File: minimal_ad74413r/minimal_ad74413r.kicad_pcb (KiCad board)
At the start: 4 copper layers, 30.5 x 25.4 mm, 17 parts, among them U8 AD74413RBCPZ

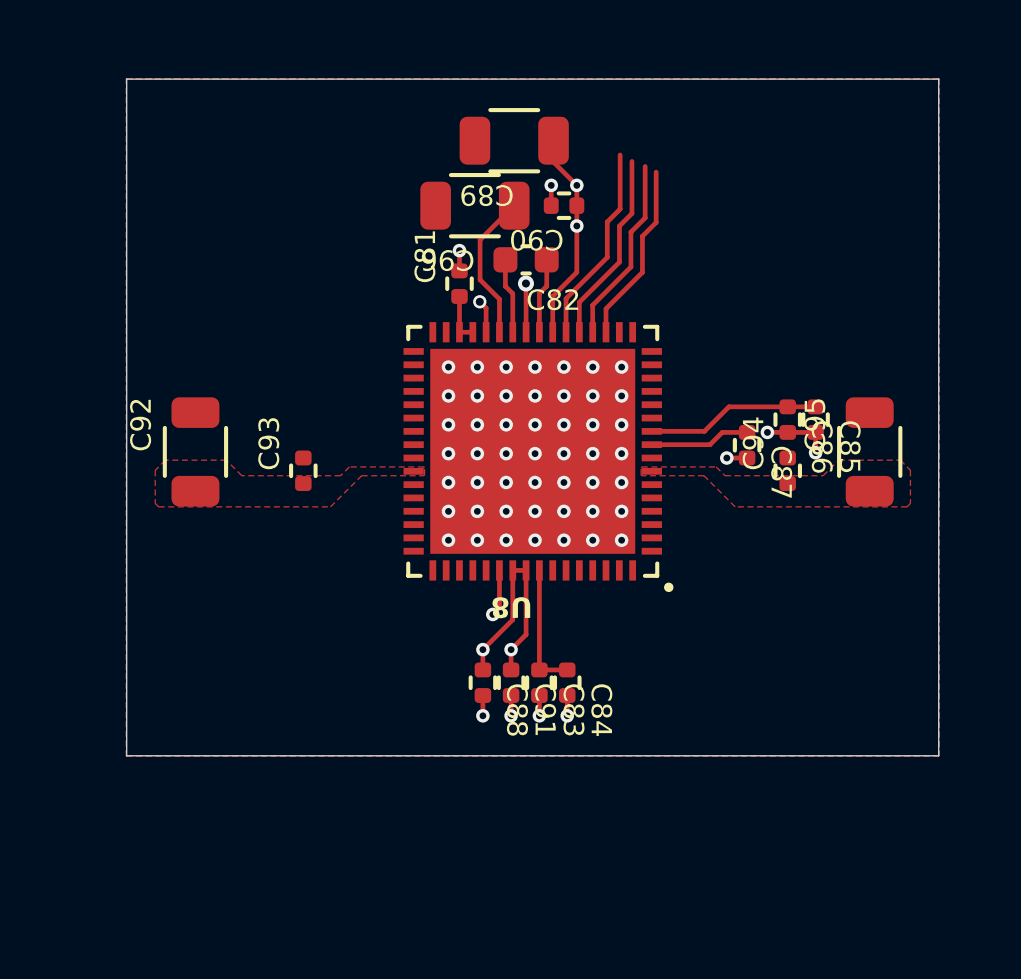
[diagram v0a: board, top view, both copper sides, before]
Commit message: backup
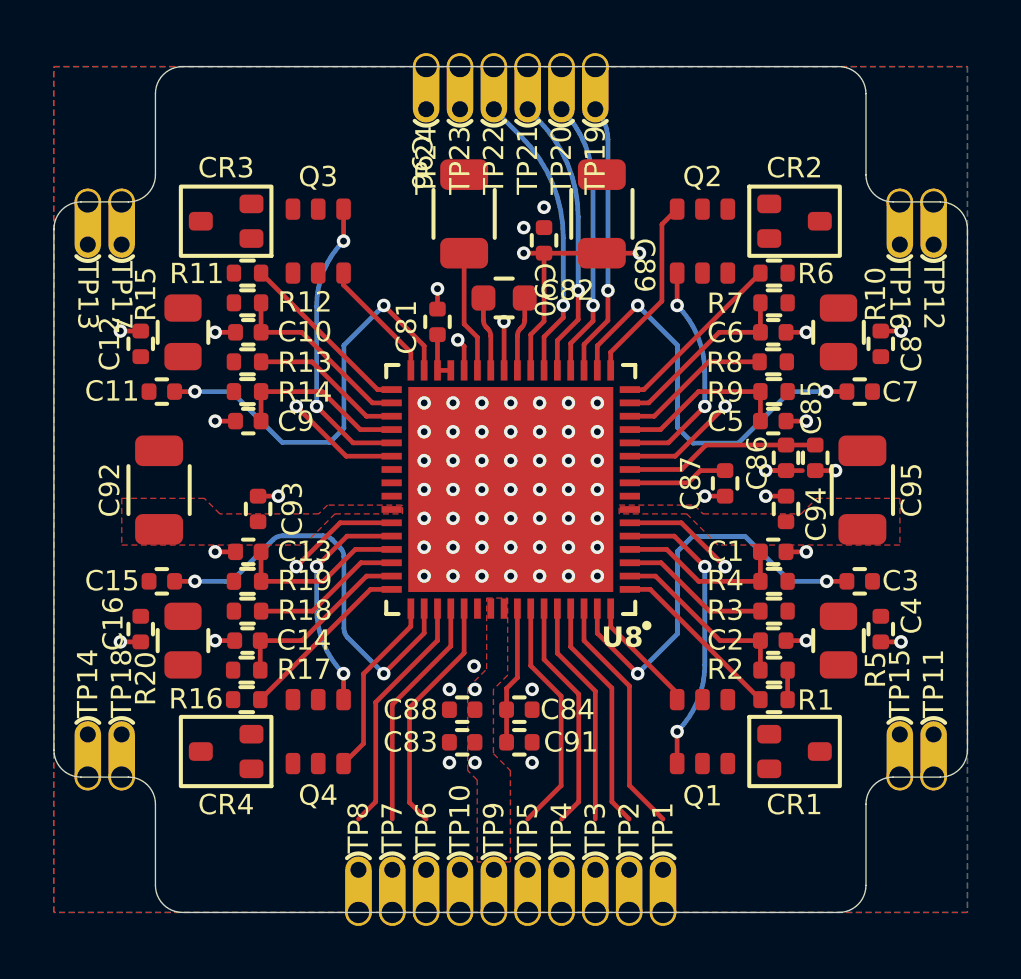
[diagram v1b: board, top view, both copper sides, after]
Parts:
- added C1: 0.01 uF, capacitor_footprints:C_0402_1005Metric, F.Cu at (161.6, 105.2)
- added C10: 0.01 uF, capacitor_footprints:C_0402_1005Metric, F.Cu at (141.9, 97.0)
- added C11: 220 pF, capacitor_footprints:C_0402_1005Metric, F.Cu at (138.7, 99.2)
- added C12: 0.01 uF, capacitor_footprints:C_0402_1005Metric, F.Cu at (137.9, 97.4)
- added C13: 0.01 uF, capacitor_footprints:C_0402_1005Metric, F.Cu at (141.9, 105.2)
- added C14: 0.01 uF, capacitor_footprints:C_0402_1005Metric, F.Cu at (141.9, 108.5)
- added C15: 220 pF, capacitor_footprints:C_0402_1005Metric, F.Cu at (138.7, 106.3)
- added C16: 0.01 uF, capacitor_footprints:C_0402_1005Metric, F.Cu at (137.9, 108.1)
- added C2: 0.01 uF, capacitor_footprints:C_0402_1005Metric, F.Cu at (161.6, 108.5)
- added C3: 220 pF, capacitor_footprints:C_0402_1005Metric, F.Cu at (164.9, 106.3)
- added C4: 0.01 uF, capacitor_footprints:C_0402_1005Metric, F.Cu at (165.7, 108.1)
- added C5: 0.01 uF, capacitor_footprints:C_0402_1005Metric, F.Cu at (161.6, 100.3)
- added C6: 0.01 uF, capacitor_footprints:C_0402_1005Metric, F.Cu at (161.6, 97.0)
- added C7: 220 pF, capacitor_footprints:C_0402_1005Metric, F.Cu at (164.9, 99.2)
- added C8: 0.01 uF, capacitor_footprints:C_0402_1005Metric, F.Cu at (165.7, 97.4)
- added C9: 0.01 uF, capacitor_footprints:C_0402_1005Metric, F.Cu at (141.9, 100.3)
- added CR1: SBAV99WT1G, diode_footprints:SC_70, F.Cu at (162.4, 112.7)
- added CR2: SBAV99WT1G, diode_footprints:SC_70, F.Cu at (162.4, 92.8)
- added CR3: SBAV99WT1G, diode_footprints:SC_70, F.Cu at (141.1, 92.8)
- added CR4: SBAV99WT1G, diode_footprints:SC_70, F.Cu at (141.1, 112.7)
- added Q1: ZXMP6A17E6TA, transistor_footprints:SOT-26, F.Cu at (159.0, 112.0)
- added Q2: ZXMP6A17E6TA, transistor_footprints:SOT-26, F.Cu at (159.0, 93.5)
- added Q3: ZXMP6A17E6TA, transistor_footprints:SOT-26, F.Cu at (144.5, 93.5)
- added Q4: ZXMP6A17E6TA, transistor_footprints:SOT-26, F.Cu at (144.5, 112.0)
- added R1: 2k, resistor_footprints:R_0402_1005Metric, F.Cu at (161.6, 110.8)
- added R10: 100, resistor_footprints:R_0805_2012Metric, F.Cu at (164.1, 97.0)
- added R11: 2k, resistor_footprints:R_0402_1005Metric, F.Cu at (141.9, 94.7)
- added R12: 10k, resistor_footprints:R_0402_1005Metric, F.Cu at (141.9, 95.9)
- added R13: 2k, resistor_footprints:R_0402_1005Metric, F.Cu at (141.9, 98.1)
- added R14: 10k, resistor_footprints:R_0402_1005Metric, F.Cu at (141.9, 99.2)
- added R15: 100, resistor_footprints:R_0805_2012Metric, F.Cu at (139.5, 97.0)
- added R16: 2k, resistor_footprints:R_0402_1005Metric, F.Cu at (141.9, 110.8)
- added R17: 10k, resistor_footprints:R_0402_1005Metric, F.Cu at (141.9, 109.6)
- added R18: 2k, resistor_footprints:R_0402_1005Metric, F.Cu at (141.9, 107.4)
- added R19: 10k, resistor_footprints:R_0402_1005Metric, F.Cu at (141.9, 106.3)
- added R2: 10k, resistor_footprints:R_0402_1005Metric, F.Cu at (161.6, 109.6)
- added R20: 100, resistor_footprints:R_0805_2012Metric, F.Cu at (139.5, 108.5)
- added R3: 2k, resistor_footprints:R_0402_1005Metric, F.Cu at (161.6, 107.4)
- added R4: 10k, resistor_footprints:R_0402_1005Metric, F.Cu at (161.6, 106.3)
- added R5: 100, resistor_footprints:R_0805_2012Metric, F.Cu at (164.1, 108.5)
- added R6: 2k, resistor_footprints:R_0402_1005Metric, F.Cu at (161.6, 94.7)
- added R7: 10k, resistor_footprints:R_0402_1005Metric, F.Cu at (161.6, 95.9)
- added R8: 2k, resistor_footprints:R_0402_1005Metric, F.Cu at (161.6, 98.1)
- added R9: 10k, resistor_footprints:R_0402_1005Metric, F.Cu at (161.6, 99.2)
- added TP1: TestPoint, test_point_footprints:TestPoint_THTPad_Castelated, F.Cu at (157.5, 118.7)
- added TP10: TestPoint, test_point_footprints:TestPoint_THTPad_Castelated, F.Cu at (149.9, 118.7)
- added TP11: TestPoint, test_point_footprints:TestPoint_THTPad_Castelated, F.Cu at (167.6, 113.7)
- added TP12: TestPoint, test_point_footprints:TestPoint_THTPad_Castelated, F.Cu at (167.6, 92.1)
- added TP13: TestPoint, test_point_footprints:TestPoint_THTPad_Castelated, F.Cu at (135.9, 92.1)
- added TP14: TestPoint, test_point_footprints:TestPoint_THTPad_Castelated, F.Cu at (135.9, 113.7)
- added TP15: TestPoint, test_point_footprints:TestPoint_THTPad_Castelated, F.Cu at (166.4, 113.7)
- added TP16: TestPoint, test_point_footprints:TestPoint_THTPad_Castelated, F.Cu at (166.4, 92.1)
- added TP17: TestPoint, test_point_footprints:TestPoint_THTPad_Castelated, F.Cu at (137.2, 92.1)
- added TP18: TestPoint, test_point_footprints:TestPoint_THTPad_Castelated, F.Cu at (137.2, 113.7)
- added TP19: TestPoint, test_point_footprints:TestPoint_THTPad_Castelated, F.Cu at (154.9, 87.0)
- added TP2: TestPoint, test_point_footprints:TestPoint_THTPad_Castelated, F.Cu at (156.2, 118.7)
- added TP20: TestPoint, test_point_footprints:TestPoint_THTPad_Castelated, F.Cu at (153.7, 87.0)
- added TP21: TestPoint, test_point_footprints:TestPoint_THTPad_Castelated, F.Cu at (152.4, 87.0)
- added TP22: TestPoint, test_point_footprints:TestPoint_THTPad_Castelated, F.Cu at (151.1, 87.0)
- added TP23: TestPoint, test_point_footprints:TestPoint_THTPad_Castelated, F.Cu at (149.9, 87.0)
- added TP24: TestPoint, test_point_footprints:TestPoint_THTPad_Castelated, F.Cu at (148.6, 87.0)
- added TP3: TestPoint, test_point_footprints:TestPoint_THTPad_Castelated, F.Cu at (154.9, 118.7)
- added TP4: TestPoint, test_point_footprints:TestPoint_THTPad_Castelated, F.Cu at (153.7, 118.7)
- added TP5: TestPoint, test_point_footprints:TestPoint_THTPad_Castelated, F.Cu at (152.4, 118.7)
- added TP6: TestPoint, test_point_footprints:TestPoint_THTPad_Castelated, F.Cu at (148.6, 118.7)
- added TP7: TestPoint, test_point_footprints:TestPoint_THTPad_Castelated, F.Cu at (147.3, 118.7)
- added TP8: TestPoint, test_point_footprints:TestPoint_THTPad_Castelated, F.Cu at (146.1, 118.7)
- added TP9: TestPoint, test_point_footprints:TestPoint_THTPad_Castelated, F.Cu at (151.1, 118.7)
- C82: footprint footprints:C_0603_1608Metric -> capacitor_footprints:C_0603_1608Metric
- moved C89 4.29 mm to (155.2, 92.5), turned to 90 degrees
- moved C91 2.89 mm to (149.9, 112.4), turned to 180 degrees
- moved C83 2.36 mm to (152.1, 112.4), turned to 0 degrees
- moved C93 2.22 mm to (142.3, 103.6)
- moved C84 2.06 mm to (152.1, 111.1), turned to 0 degrees
- moved C92 1.98 mm to (138.6, 102.9)
- moved U8 1.65 mm to (151.8, 102.9)
- moved C81 1.65 mm to (149.0, 96.6)
- moved C82 1.65 mm to (151.5, 95.7)
- moved C87 1.65 mm to (159.8, 102.6)
- moved C90 1.50 mm to (153.0, 93.5), turned to 90 degrees
- moved C95 1.46 mm to (165.0, 102.9)
- moved C86 1.43 mm to (162.1, 101.7)
- moved C94 1.43 mm to (162.1, 103.6)
- moved C85 1.43 mm to (163.2, 101.7)
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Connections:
- C88 pad 1: (no net) -> /3V3
- C89 pad 1: /3V3_ISO -> /3V3
- C90 pad 1: /3V3_ISO -> /3V3
- C91 pad 1: (no net) -> /3V3
- U8 pad 23: /3V3_ISO -> /3V3
- U8 pad 28: (no net) -> GNDA
- U8 pad 55: (no net) -> /3V3
- U8 pad 56: (no net) -> /3V3
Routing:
- net /3V3_ISO: track 16.6 -> 0.00 mm, vias 4 -> 0
- net /CCOMP_B: track 0.00 -> 15.7 mm, vias 0 -> 2
- net /CCOMP_C: track 0.00 -> 15.7 mm, vias 0 -> 2
- net /CCOMP_A: track 0.00 -> 15.6 mm, vias 0 -> 2
- net /CCOMP_D: track 0.00 -> 15.5 mm, vias 0 -> 2
- net /VIOUTP_C: track 0.00 -> 11.0 mm, vias 0 -> 2
- net /VIOUTP_A: track 0.00 -> 10.9 mm, vias 0 -> 2
- net /SDO: track 0.00 -> 9.13 mm
- net /~{RESET}: track 0.00 -> 9.13 mm
- net /~{ALERT}: track 0.00 -> 9.01 mm
- net /3V3: track 0.00 -> 8.95 mm, vias 0 -> 4
- net /~{LDAC}: track 0.00 -> 8.89 mm
- net /~{ADC_RDY}: track 0.00 -> 8.81 mm
- net /~{SYNC}: track 0.00 -> 8.81 mm
- net /SCLK: track 0.00 -> 8.71 mm
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- added copper zone on F.Cu, net /3V3
- added copper zone on In1.Cu, net /VDD_24V
- added copper zone on In1.Cu, net GNDA
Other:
- board size 30.5 x 25.4 mm -> 34.3 x 31.8 mm
